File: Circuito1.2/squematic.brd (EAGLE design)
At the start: 65.7 x 55.9 mm, 24 parts, among them IC1 LM358N

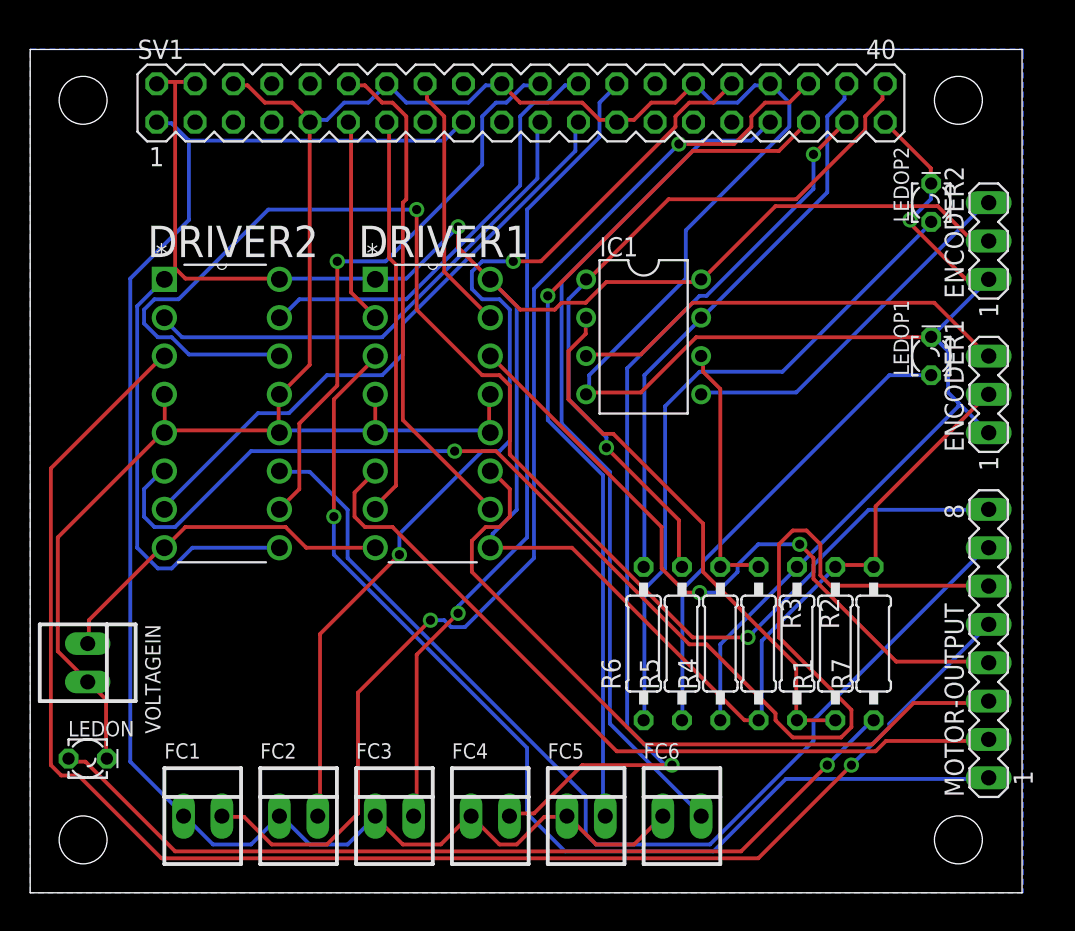
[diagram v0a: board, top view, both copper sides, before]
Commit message: PCB Fischer FINAL Subido a PCBWAY
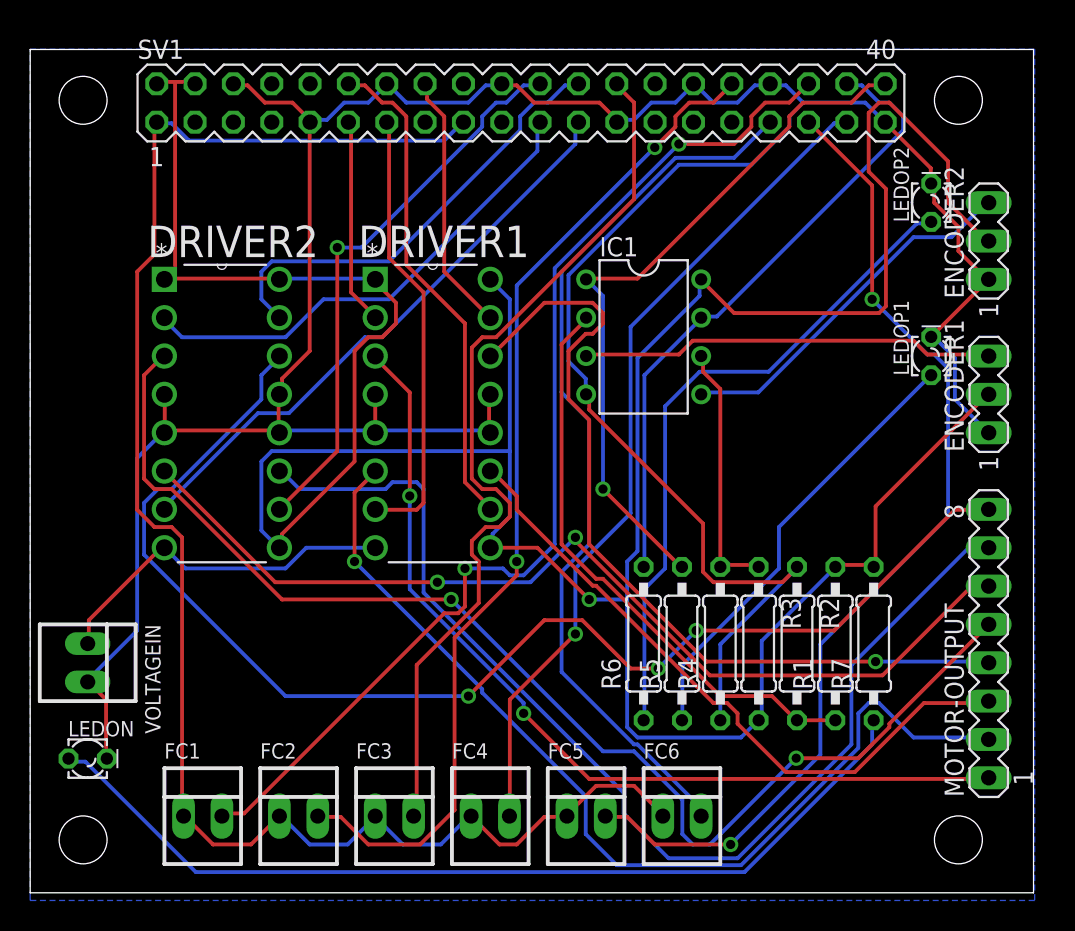
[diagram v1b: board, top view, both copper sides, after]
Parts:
- R5, R6: value 3k9 -> 330
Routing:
- net +5V: track 180.2 -> 216.1 mm
- net M3-: track 92.4 -> 65.3 mm, vias 1 -> 2
- net M3+: track 101.5 -> 82.2 mm, vias 1 -> 2
- net M1-: track 52.4 -> 65.3 mm, vias 0 -> 1
- net GND: track 226.2 -> 216.0 mm, vias 1 -> 0
- net M1+: track 70.4 -> 60.4 mm, vias 1 -> 2
- net M2-: track 46.7 -> 56.0 mm, vias 2 -> 1
- net GPIO19: track 58.1 -> 67.0 mm, vias 1 -> 2
- net GPIO26: track 62.7 -> 55.7 mm, vias 2 -> 1
- net M4-: track 91.6 -> 85.0 mm, vias 2 -> 3
- net GPIO7: track 54.1 -> 59.1 mm, vias 1 -> 0
- net M4+: track 69.5 -> 74.4 mm
- net M2+: track 49.0 -> 44.1 mm
- net GPIO20: track 37.6 -> 42.1 mm
- net GPIO16: track 76.4 -> 71.9 mm
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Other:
- board size 65.7 x 55.9 mm -> 66.5 x 55.9 mm
